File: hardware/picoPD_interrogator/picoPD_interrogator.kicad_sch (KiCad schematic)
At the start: 25 parts, among them Q1 rohm-RE1C002UN, Q2 rohm-RE1C002UN, Q3 rohm-RE1C002UN, Q4 rohm-RE1C002UN, U2 ST-LM393QT

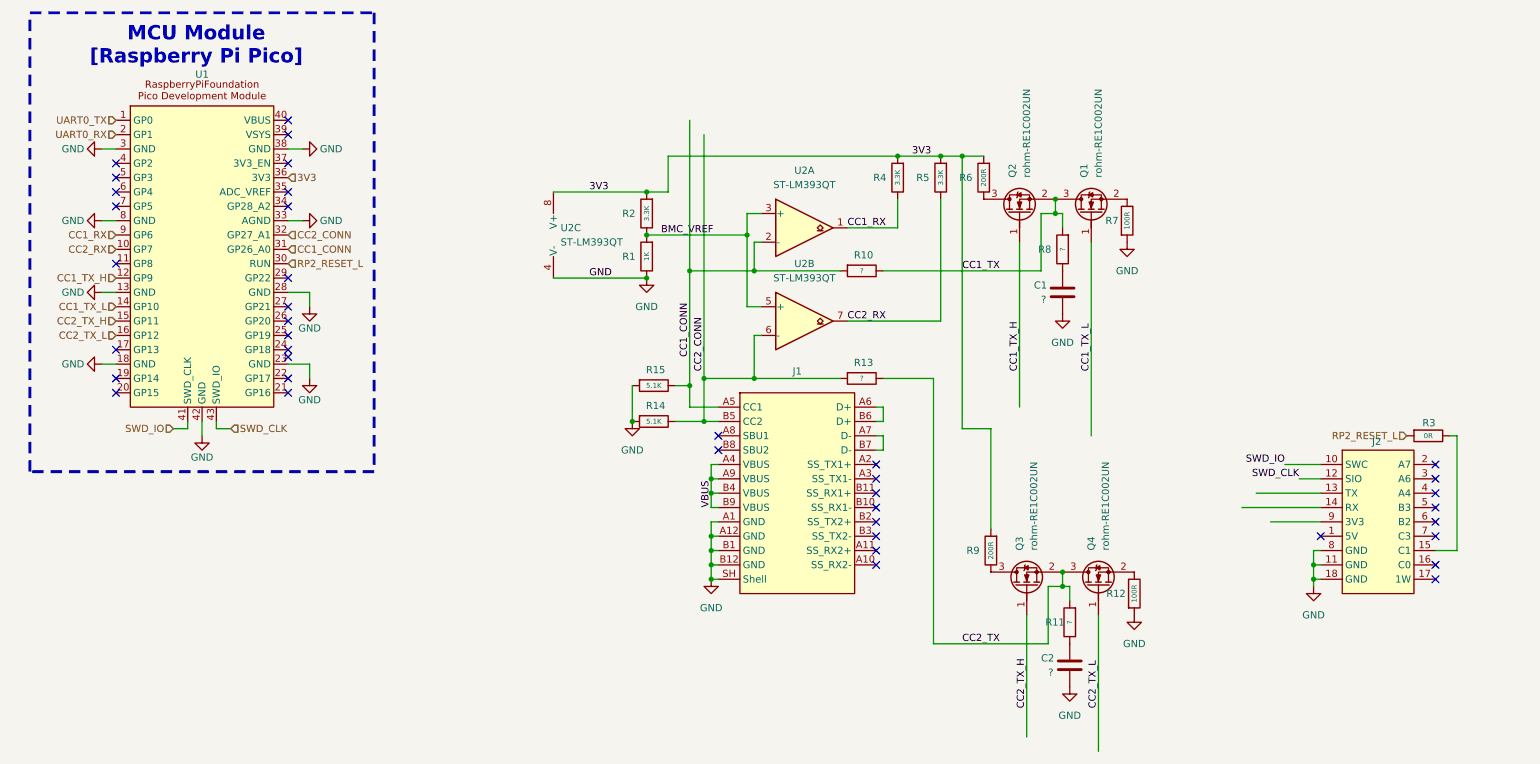
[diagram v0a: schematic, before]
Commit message: Cleaned up schematic layout.
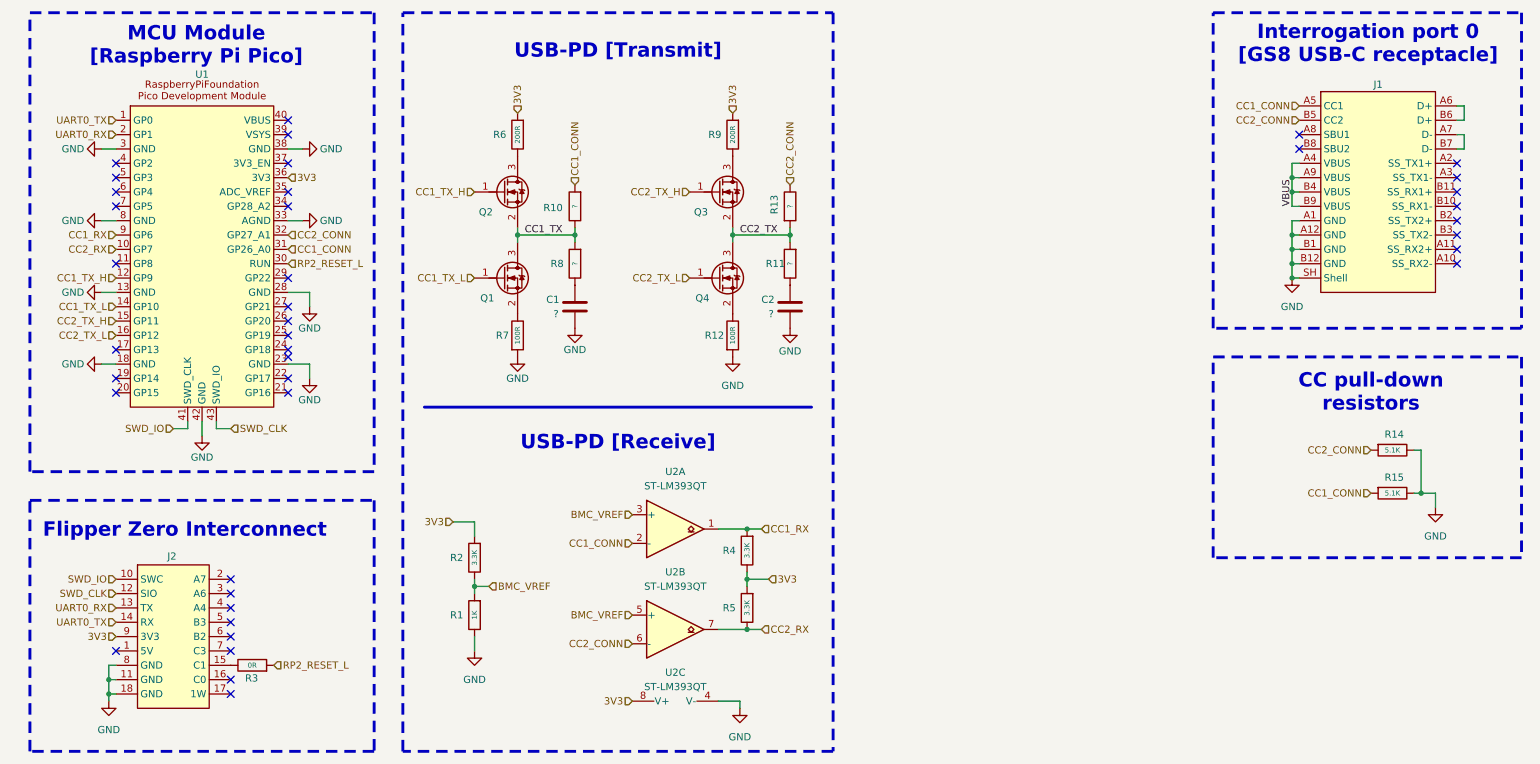
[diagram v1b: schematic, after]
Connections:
- net 3V3: now also J2.9 (3V3), R4.1; no longer Q1.3 (D), Q2.2 (S), R10.1, R4.2, R8.2
- net CC1_CONN: now also R15.2; no longer R15.1
- net CC1_RX: now also R4.2; no longer R4.1
- net CC2_CONN: now also R13.1, R14.2; no longer R13.2, R14.1
- net CC2_TX: now also R13.2; no longer R13.1
- net GND: now also R14.1, R15.1; no longer R14.2, R15.2
- net UART0_RX: now also J2.13 (TX)
- net UART0_TX: now also J2.14 (RX)
- new net CC1_TX: Q1.3 (D), Q2.2 (S), R10.1, R8.2
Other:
- note added: "CC pull-down resistors"
- note added: "Flipper Zero Interconnect"
- note added: "Interrogation port 0 [GS8 USB-C receptacle]"
- note added: "USB-PD [Receive]"
- note added: "USB-PD [Transmit]"
- moved on the sheet: C1, C2, J1, J2, Q1, Q2, Q3, Q4, R1, R10, R11, R12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
